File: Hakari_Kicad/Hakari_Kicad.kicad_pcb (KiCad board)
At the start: 2 copper layers, 70.5 x 83 mm, 5 parts, among them U2 MP6500

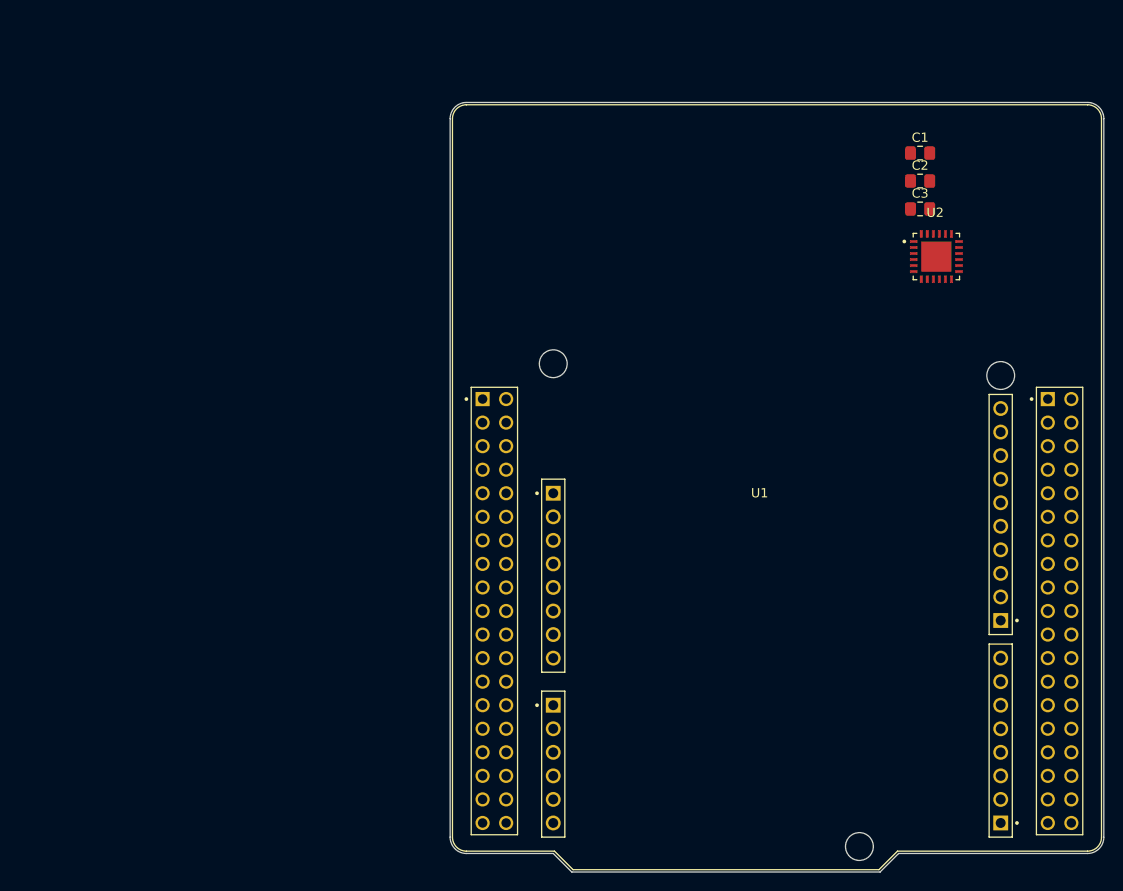
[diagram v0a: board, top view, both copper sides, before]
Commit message: Hakari PCB
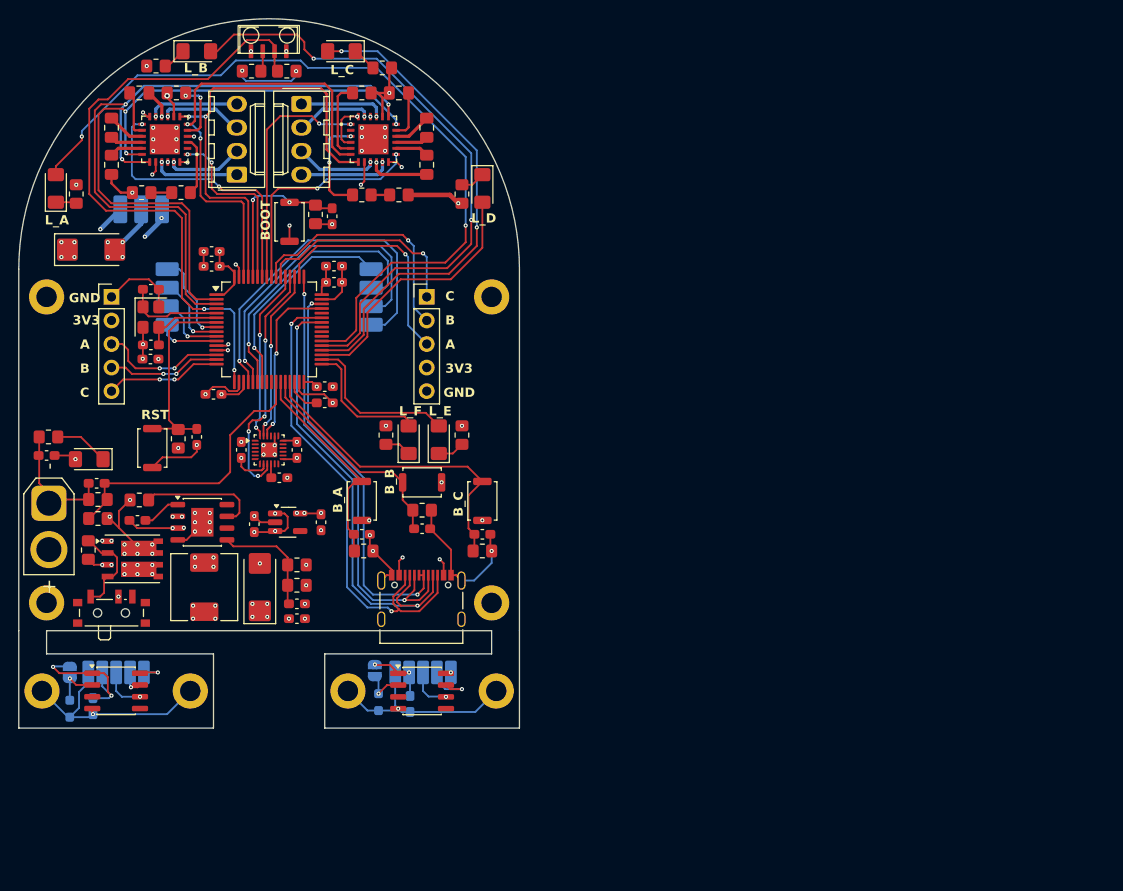
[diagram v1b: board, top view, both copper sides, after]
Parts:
- added C10: 100nF, Capacitor_SMD:C_0603_1608Metric_Pad1.08x0.95mm_HandSolder, F.Cu at (97.0, 100.0)
- added C11: 100nF, Capacitor_SMD:C_0603_1608Metric_Pad1.08x0.95mm_HandSolder, F.Cu at (106.0, 93.2)
- added C12: 100nF, Capacitor_SMD:C_0603_1608Metric_Pad1.08x0.95mm_HandSolder, F.Cu at (93.8, 80.2)
- added C13: 100nF, Capacitor_SMD:C_0603_1608Metric_Pad1.08x0.95mm_HandSolder, F.Cu at (107.0, 80.2)
- added C14: 100nF, Capacitor_SMD:C_0603_1608Metric_Pad1.08x0.95mm_HandSolder, F.Cu at (87.2, 90.2)
- added C15: 100nF, Capacitor_SMD:C_0603_1608Metric_Pad1.08x0.95mm_HandSolder, F.Cu at (94.0, 94.0)
- added C16: 4.7uF, Capacitor_SMD:C_0603_1608Metric_Pad1.08x0.95mm_HandSolder, F.Cu at (107.0, 81.9)
- added C17: 1uF, Capacitor_SMD:C_0603_1608Metric_Pad1.08x0.95mm_HandSolder, F.Cu at (93.8, 78.6)
- added C18: 100nF, Capacitor_SMD:C_0805_2012Metric_Pad1.18x1.45mm_HandSolder, F.Cu at (117.0, 65.2)
- added C19: 100nF, Capacitor_SMD:C_0805_2012Metric_Pad1.18x1.45mm_HandSolder, F.Cu at (117.0, 69.2)
- added C20: 220nF, Capacitor_SMD:C_0805_2012Metric_Pad1.18x1.45mm_HandSolder, F.Cu at (114.0, 61.5)
- added C21: 100nF, Capacitor_SMD:C_0805_2012Metric_Pad1.18x1.45mm_HandSolder, F.Cu at (83.0, 65.2)
- added C22: 220nF, Capacitor_SMD:C_0805_2012Metric_Pad1.18x1.45mm_HandSolder, F.Cu at (83.0, 69.2)
- added C23: 100nF, Capacitor_SMD:C_0805_2012Metric_Pad1.18x1.45mm_HandSolder, F.Cu at (86.0, 61.5)
- added C24: 10nF, Capacitor_SMD:C_0603_1608Metric_Pad1.08x0.95mm_HandSolder, F.Cu at (123.0, 109.1)
- added C29: 10uF, Capacitor_Tantalum_SMD:CP_EIA-6032-15_Kemet-U_HandSolder, F.Cu at (80.8, 78.4)
- added C30: 100nF, Capacitor_SMD:C_0603_1608Metric_Pad1.08x0.95mm_HandSolder, F.Cu at (76.0, 100.6)
- added C31: 100nF, Capacitor_SMD:C_0603_1608Metric_Pad1.08x0.95mm_HandSolder, F.Cu at (85.8, 107.6)
- added C32: 1uF, Capacitor_SMD:C_0603_1608Metric_Pad1.08x0.95mm_HandSolder, F.Cu at (98.4, 108.0)
- added C33: 1uF, Capacitor_SMD:C_0603_1608Metric_Pad1.08x0.95mm_HandSolder, F.Cu at (105.6, 107.8)
- added C34: 100nF, Capacitor_SMD:C_0603_1608Metric_Pad1.08x0.95mm_HandSolder, F.Cu at (103.0, 116.6)
- added C35: 100nF, Capacitor_SMD:C_0603_1608Metric_Pad1.08x0.95mm_HandSolder, F.Cu at (103.0, 118.2)
- added C37: 100uF, Capacitor_Tantalum_SMD:CP_EIA-6032-15_Kemet-U_HandSolder, F.Cu at (99.0, 114.8)
- added C39: 100nF, Capacitor_SMD:C_0603_1608Metric_Pad1.08x0.95mm_HandSolder, B.Cu at (81.0, 127.6)
- added C4: 10nF, Capacitor_SMD:C_0603_1608Metric_Pad1.08x0.95mm_HandSolder, F.Cu at (106.8, 74.8)
- added C41: 100nF, Capacitor_SMD:C_0603_1608Metric_Pad1.08x0.95mm_HandSolder, B.Cu at (115.2, 127.4)
- added C44: 100nF, Capacitor_SMD:C_0603_1608Metric_Pad1.08x0.95mm_HandSolder, F.Cu at (81.4, 103.6)
- added C5: 4.7uF, Capacitor_SMD:C_0603_1608Metric_Pad1.08x0.95mm_HandSolder, F.Cu at (106.0, 94.9)
- added C6: 10nF, Capacitor_SMD:C_0603_1608Metric_Pad1.08x0.95mm_HandSolder, F.Cu at (103.0, 100.0)
- added C7: 20pF, Capacitor_SMD:C_0603_1608Metric_Pad1.08x0.95mm_HandSolder, F.Cu at (87.2, 82.7)
- added C8: 100nF, Capacitor_SMD:C_0603_1608Metric_Pad1.08x0.95mm_HandSolder, F.Cu at (101.1, 103.0)
- added C9: 20pF, Capacitor_SMD:C_0603_1608Metric_Pad1.08x0.95mm_HandSolder, F.Cu at (87.2, 88.7)
- added D10: LED, LED_SMD:LED_1206_3216Metric_Pad1.42x1.75mm_HandSolder, F.Cu at (80.6, 101.0)
- added D2: LED, LED_SMD:LED_1206_3216Metric_Pad1.42x1.75mm_HandSolder, F.Cu at (77.0, 71.8)
- added D3: LED, LED_SMD:LED_1206_3216Metric_Pad1.42x1.75mm_HandSolder, F.Cu at (92.2, 57.0)
- added D4: LED, LED_SMD:LED_1206_3216Metric_Pad1.42x1.75mm_HandSolder, F.Cu at (107.8, 57.0)
- added D5: LED, LED_SMD:LED_1206_3216Metric_Pad1.42x1.75mm_HandSolder, F.Cu at (123.0, 71.8)
- added D6: LED, LED_SMD:LED_1206_3216Metric_Pad1.42x1.75mm_HandSolder, F.Cu at (118.3, 98.9)
- added D7: LED, LED_SMD:LED_1206_3216Metric_Pad1.42x1.75mm_HandSolder, F.Cu at (115.0, 98.9)
- added H10: MountingHole_Pad, MountingHole:MountingHole_2.2mm_M2_ISO14580_Pad, F.Cu at (75.5, 126.0)
- added H11: MountingHole_Pad, MountingHole:MountingHole_2.2mm_M2_ISO14580_Pad, F.Cu at (124.5, 126.0)
- added H12: MountingHole_Pad, MountingHole:MountingHole_2.2mm_M2_ISO14580_Pad, F.Cu at (108.5, 126.0)
- added H5: MountingHole_Pad, MountingHole:MountingHole_2.2mm_M2_ISO14580_Pad, F.Cu at (76.0, 116.5)
- added H6: MountingHole_Pad, MountingHole:MountingHole_2.2mm_M2_ISO14580_Pad, F.Cu at (124.0, 116.5)
- added H7: MountingHole_Pad, MountingHole:MountingHole_2.2mm_M2_ISO14580_Pad, F.Cu at (124.0, 83.5)
- added H8: MountingHole_Pad, MountingHole:MountingHole_2.2mm_M2_ISO14580_Pad, F.Cu at (76.0, 83.5)
- added H9: MountingHole_Pad, MountingHole:MountingHole_2.2mm_M2_ISO14580_Pad, F.Cu at (91.5, 126.0)
- added J1: MR, Connector_Molex:Molex_KK-254_AE-6410-04A_1x04_P2.54mm_Vertical, F.Cu at (103.5, 62.7)
- added J11: XT30_BATT, Connector_AMASS:AMASS_XT30U-F_1x02_P5.0mm_Vertical, F.Cu at (76.2, 105.8)
- added J13: SQJ951EP, Package_SO:PowerPAK_SO-8_Dual, F.Cu at (85.2, 111.8)
- added J15: ~, Footprint:AS5145_Mod, B.Cu at (83.5, 124.0)
- added J16: ~, Footprint:AS5145_Mod, B.Cu at (116.6, 124.0)
- added J2: ~, Footprint:usb_C_stm32, F.Cu at (116.4, 113.6)
- added J3: ML, Connector_Molex:Molex_KK-254_AE-6410-04A_1x04_P2.54mm_Vertical, F.Cu at (96.5, 70.3)
- added J4: ~, Connector_PinHeader_2.54mm:PinHeader_1x05_P2.54mm_Vertical, F.Cu at (83.0, 83.5)
- added J5: ~, Connector_PinHeader_2.54mm:PinHeader_1x05_P2.54mm_Vertical, F.Cu at (117.0, 83.5)
- added J6: IR_TX, Footprint:CONN_SMD_01X04_IR, B.Cu at (89.0, 83.5)
- added J7: IR_RX, Footprint:CONN_SMD_01X04_IR, B.Cu at (111.0, 83.5)
- added J8: VCC_IR, Footprint:CONN_SMD_01X03_IR, B.Cu at (86.2, 73.8)
- added JP1: Jumper_2_Open, Jumper:SolderJumper-2_P1.3mm_Open_RoundedPad1.0x1.5mm, B.Cu at (78.5, 124.0)
- added JP2: Jumper_2_Open, Jumper:SolderJumper-2_P1.3mm_Open_RoundedPad1.0x1.5mm, B.Cu at (111.4, 123.8)
- added L1: 4.7uH, Inductor_SMD:L_Wuerth_HCM-7050, F.Cu at (93.0, 114.8)
- added R11: 220, Resistor_SMD:R_0805_2012Metric_Pad1.20x1.40mm_HandSolder, F.Cu at (79.2, 72.4)
- added R12: 220, Resistor_SMD:R_0805_2012Metric_Pad1.20x1.40mm_HandSolder, F.Cu at (87.8, 58.6)
- added R13: 220, Resistor_SMD:R_0805_2012Metric_Pad1.20x1.40mm_HandSolder, F.Cu at (112.2, 58.8)
- added R14: 220, Resistor_SMD:R_0805_2012Metric_Pad1.20x1.40mm_HandSolder, F.Cu at (120.8, 72.4)
- added R15: 82k, Resistor_SMD:R_0805_2012Metric_Pad1.20x1.40mm_HandSolder, F.Cu at (81.5, 107.4)
- added R16: 39K, Resistor_SMD:R_0805_2012Metric_Pad1.20x1.40mm_HandSolder, F.Cu at (81.5, 105.3)
- added R17: 220, Resistor_SMD:R_0805_2012Metric_Pad1.20x1.40mm_HandSolder, F.Cu at (120.8, 98.4)
- added R18: 220, Resistor_SMD:R_0805_2012Metric_Pad1.20x1.40mm_HandSolder, F.Cu at (112.6, 98.4)
- added R19: 220k, Resistor_SMD:R_0805_2012Metric_Pad1.20x1.40mm_HandSolder, F.Cu at (110.0, 61.5)
- added R2: 10K, Resistor_SMD:R_0805_2012Metric_Pad1.20x1.40mm_HandSolder, F.Cu at (90.2, 98.8)
- added R20: 100k, Resistor_SMD:R_0805_2012Metric_Pad1.20x1.40mm_HandSolder, F.Cu at (110.0, 72.5)
- added R21: 18k, Resistor_SMD:R_0805_2012Metric_Pad1.20x1.40mm_HandSolder, F.Cu at (114.0, 72.5)
- added R22: 100k, Resistor_SMD:R_0805_2012Metric_Pad1.20x1.40mm_HandSolder, F.Cu at (90.5, 72.2)
- added R23: 18k, Resistor_SMD:R_0805_2012Metric_Pad1.20x1.40mm_HandSolder, F.Cu at (86.2, 72.2)
- added R24: 220k, Resistor_SMD:R_0805_2012Metric_Pad1.20x1.40mm_HandSolder, F.Cu at (90.0, 61.5)
- added R3: 10K, Resistor_SMD:R_0805_2012Metric_Pad1.20x1.40mm_HandSolder, F.Cu at (110.2, 110.9)
- added R4: 10K, Resistor_SMD:R_0805_2012Metric_Pad1.20x1.40mm_HandSolder, F.Cu at (101.9, 59.1)
- added R5: 100, Resistor_SMD:R_0805_2012Metric_Pad1.20x1.40mm_HandSolder, F.Cu at (98.1, 59.1)
- added R56: 220, Resistor_SMD:R_0805_2012Metric_Pad1.20x1.40mm_HandSolder, F.Cu at (76.2, 98.6)
- added R57: 100k, Resistor_SMD:R_0805_2012Metric_Pad1.20x1.40mm_HandSolder, F.Cu at (80.5, 110.8)
- added R58: 10K, Resistor_SMD:R_0805_2012Metric_Pad1.20x1.40mm_HandSolder, F.Cu at (86.0, 105.4)
- added R59: 44K, Resistor_SMD:R_0805_2012Metric_Pad1.20x1.40mm_HandSolder, F.Cu at (103.0, 114.6)
- added R6: 10K, Resistor_SMD:R_0805_2012Metric_Pad1.20x1.40mm_HandSolder, F.Cu at (116.5, 106.5)
- added R60: 10K, Resistor_SMD:R_0805_2012Metric_Pad1.20x1.40mm_HandSolder, F.Cu at (103.0, 112.4)
- added R61: 10k, Resistor_SMD:R_0603_1608Metric_Pad0.98x0.95mm_HandSolder, B.Cu at (78.5, 127.9)
- added R62: 10k, Resistor_SMD:R_0603_1608Metric_Pad0.98x0.95mm_HandSolder, B.Cu at (111.8, 127.2)
- added R7: 10K, Resistor_SMD:R_0805_2012Metric_Pad1.20x1.40mm_HandSolder, F.Cu at (105.0, 74.6)
- added R8: 10K, Resistor_SMD:R_0805_2012Metric_Pad1.20x1.40mm_HandSolder, F.Cu at (123.0, 110.9)
- added SW1: SW_Push, Button_Switch_SMD:SW_Push_SPST_NO_Alps_SKRK, F.Cu at (87.4, 99.8)
- added SW2: SW_Push, Button_Switch_SMD:SW_Push_SPST_NO_Alps_SKRK, F.Cu at (110.0, 105.5)
- added SW3: SW_Push, Button_Switch_SMD:SW_Push_SPST_NO_Alps_SKRK, F.Cu at (116.5, 103.5)
- added SW4: SW_Push, Button_Switch_SMD:SW_Push_SPST_NO_Alps_SKRK, F.Cu at (102.2, 75.4)
- added SW5: SW_Push_SPDT, Button_Switch_SMD:SW_SPDT_PCM12, F.Cu at (83.0, 117.2)
- added SW6: SW_Push, Button_Switch_SMD:SW_Push_SPST_NO_Alps_SKRK, F.Cu at (123.0, 105.5)
- added U25: CN3903, Package_SO:HSOP-8-1EP_3.9x4.9mm_P1.27mm_EP2.41x3.1mm, F.Cu at (92.8, 107.8)
- added U26: ME6211C33_regulador, Package_TO_SOT_SMD:SOT-23-5_HandSoldering, F.Cu at (102.0, 107.8)
- added U27: MT6701CT, Package_SO:SO-8_3.9x4.9mm_P1.27mm, F.Cu at (83.5, 126.0)
- added U28: MT6701CT, Package_SO:SO-8_3.9x4.9mm_P1.27mm, F.Cu at (116.5, 126.0)
- added U3: MPU6500, Package_DFN_QFN:QFN-24-1EP_3x3mm_P0.4mm_EP1.75x1.6mm, F.Cu at (100.0, 100.0)
- added U4: MP6500, Footprint:MP6500, F.Cu at (111.2, 66.5)
- added U5: MP6500, Footprint:MP6500, F.Cu at (88.8, 66.5)
- added Y1: Crystal_GND24, Crystal:Crystal_SMD_3225-4Pin_3.2x2.5mm, F.Cu at (87.2, 85.7)
- C1: value 100nF -> 10nF; footprint Capacitor_SMD:C_0805_2012Metric_Pad1.18x1.45mm_HandSolder -> Capacitor_SMD:C_0603_1608Metric_Pad1.08x0.95mm_HandSolder
- C2: value 1uF -> 10nF; footprint Capacitor_SMD:C_0805_2012Metric_Pad1.18x1.45mm_HandSolder -> Capacitor_SMD:C_0603_1608Metric_Pad1.08x0.95mm_HandSolder
- C3: value 0.22uF -> 10nF; footprint Capacitor_SMD:C_0805_2012Metric_Pad1.18x1.45mm_HandSolder -> Capacitor_SMD:C_0603_1608Metric_Pad1.08x0.95mm_HandSolder
- U1: footprint Footprint:NUCLEO_H533 -> Footprint:IRM-V838
- U2: value MP6500 -> ~; footprint Footprint:MP6500 -> Package_QFP:LQFP-64_10x10mm_P0.5mm
- moved C1 83.8 mm to (92.2, 98.6), turned to -90 degrees
- moved U1 77.9 mm to (98.0, 57.0), turned to 90 degrees
- moved U2 72.4 mm to (100.0, 87.0)
- moved C2 71.3 mm to (110.0, 109.1)
- moved C3 63.8 mm to (116.5, 108.5)
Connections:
- C1 pad 1: Net-(U2-CP1) -> /NRST
- C1 pad 2: Net-(U2-CP2) -> GND
- C2 pad 1: Net-(C2-Pad1) -> /BOTON_A
- C2 pad 2: Net-(U2-VCP) -> GND
- C3 pad 1: Net-(U2-VG) -> /BOTON_B
- U2 pad 1: /DIR_ML -> +3.3V
- U2 pad 10: Net-(C2-Pad1) -> /IR3_TX
- U2 pad 11: Net-(J1-Pin_4) -> /IR4_TX
- U2 pad 13: /STEP_ML -> +3.3V
- U2 pad 14: Net-(U2-VCP) -> /ENCA_ML
- U2 pad 15: Net-(U2-CP2) -> /ENCB_ML
- U2 pad 16: Net-(U2-CP1) -> /ENCC_ML
- U2 pad 17: Net-(U2-VG) -> /IR_36KHZ
- U2 pad 18: /ENBL_ML -> GND
- U2 pad 19: /SLEEP_ML -> +3.3V
- U2 pad 2: Net-(U2-~FAULT) -> /ENABLE
- U2 pad 20: GND -> /IR1_RX
- U2 pad 21: Net-(J1-Pin_2) -> /IR2_RX
- U2 pad 22: Net-(C2-Pad1) -> /IR3_RX
- U2 pad 23: Net-(J1-Pin_1) -> /IR4_RX
- U2 pad 24: GND -> unconnected-(U2-PC4-Pad24)
- U2 pad 25: GND -> unconnected-(U2-PC5-Pad25)
- U2 pad 3: Net-(U2-ISET) -> /SLEEP
- U2 pad 4: GND -> unconnected-(U2-PC15_OSC32_OUT-Pad4)
- U2 pad 5: Net-(U2-ROSC) -> /OSC_A
- U2 pad 6: /MS2_ML -> /OSC_B
- U2 pad 7: /MS1_ML -> /NRST
- U2 pad 8: GND -> /IR1_TX
- U2 pad 9: Net-(J1-Pin_3) -> /IR2_TX
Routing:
- net GND: track 0.00 -> 133.4 mm, vias 0 -> 68
- net +3.3V: track 0.00 -> 97.0 mm, vias 0 -> 24
- net /LEDA: track 0.00 -> 85.9 mm, vias 0 -> 2
- net /SLEEP: track 0.00 -> 76.2 mm, vias 0 -> 3
- net /ENABLE: track 0.00 -> 72.4 mm, vias 0 -> 3
- net /IR_36KHZ: track 0.00 -> 68.8 mm, vias 0 -> 2
- net /LEDB: track 0.00 -> 67.0 mm, vias 0 -> 2
- net +5V: track 0.00 -> 55.1 mm, vias 0 -> 15
- net /LEDC: track 0.00 -> 53.8 mm, vias 0 -> 2
- net /RX: track 0.00 -> 52.6 mm, vias 0 -> 2
- net /TX: track 0.00 -> 51.0 mm, vias 0 -> 2
- net /MS1: track 0.00 -> 50.0 mm, vias 0 -> 2
- net /MS2: track 0.00 -> 49.5 mm, vias 0 -> 2
- net /SWCLK: track 0.00 -> 49.2 mm, vias 0 -> 2
- net /SWDIO: track 0.00 -> 43.2 mm, vias 0 -> 2
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- added copper zone on In2.Cu, net +3.3V
- added copper zone on In2.Cu, net +5V
- added copper zone on In2.Cu, net /VIN
- added copper zone on In1.Cu, net GND
- added copper zone on In2.Cu, net Net-(J11-VCC)
- added copper zone on In2.Cu, net Net-(U25-SW)
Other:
- board size 70.5 x 83 mm -> 54 x 76.5 mm
- copper layers 2 -> 4
- board text added: "3V3"
- board text added: "5V"
- board text added: "A"
- board text added: "B"
- board text added: "BOOT"
- board text added: "B_A"
- board text added: "B_B"
- board text added: "B_C"
- board text added: "C"
- board text added: "GND"
- board text added: "L_A"
- board text added: "L_B"
- board text added: "L_C"
- board text added: "L_D"
- board text added: "L_E"
- board text added: "L_F"
- board text added: "RST"
- board text added: "RX_1"
- board text added: "RX_2"
- board text added: "RX_3"
- board text added: "RX_4"
- board text added: "TX_1"
- board text added: "TX_2"
- board text added: "TX_3"
- board text added: "TX_4"

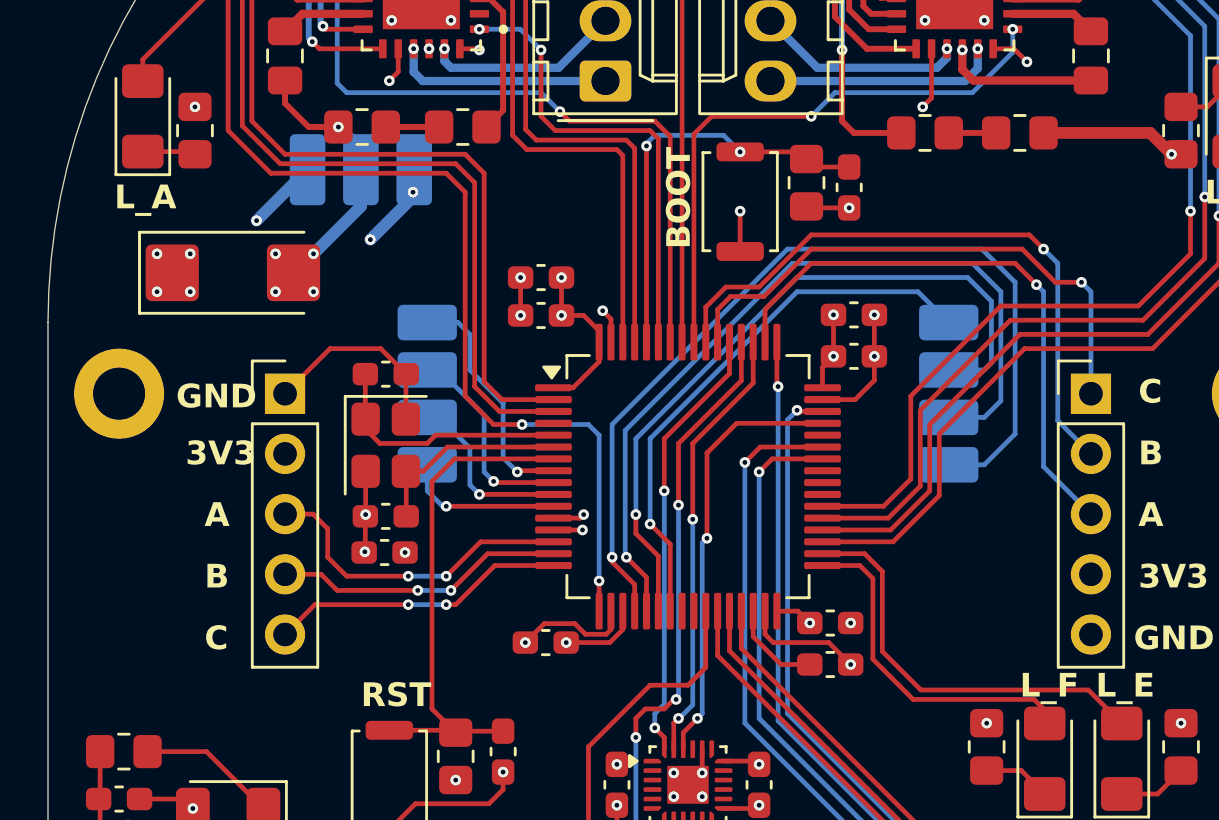
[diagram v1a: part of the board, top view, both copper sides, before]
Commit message: Agregada nueva carpeta
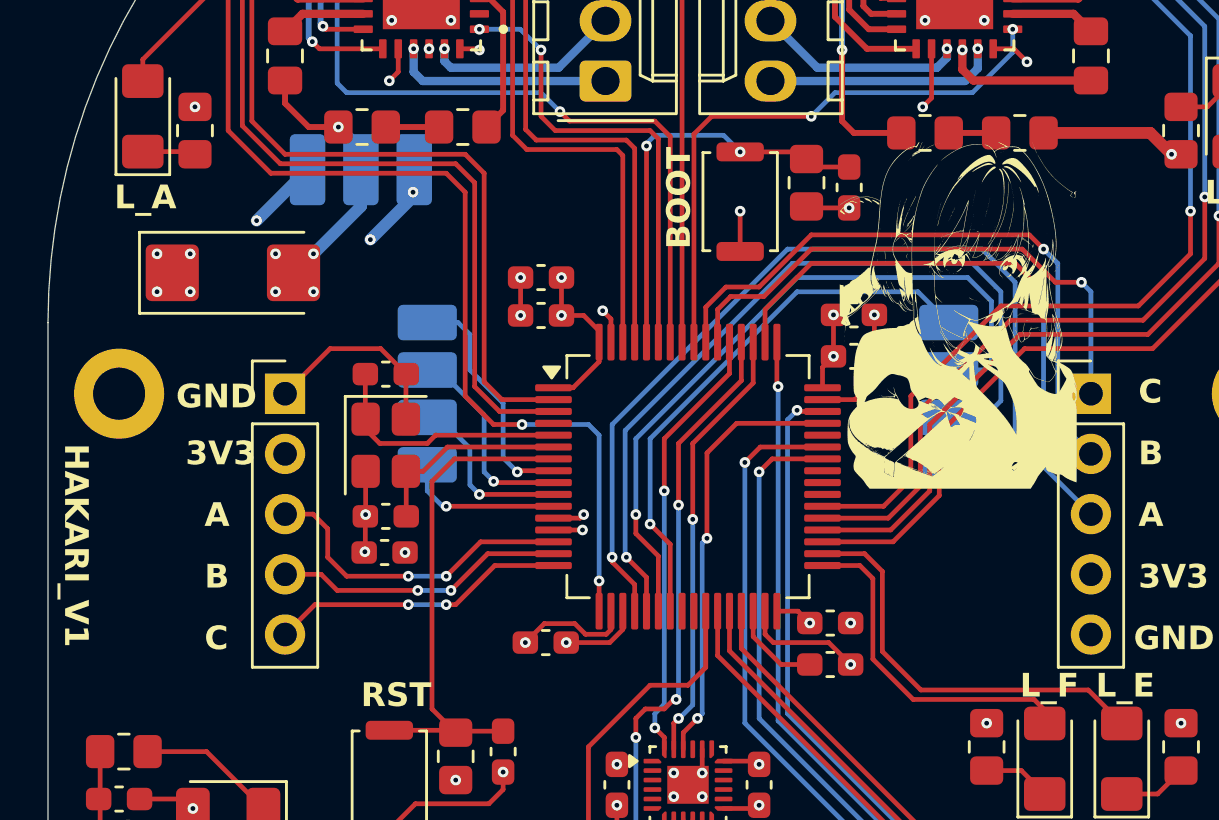
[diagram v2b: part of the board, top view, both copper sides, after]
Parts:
- added G***: LOGO, LOGO, F.Cu at (111.4, 80.2)
- added G***: LOGO, LOGO, B.Cu at (99.1, 96.4)
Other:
- board text added: "HAKARI_V1"
